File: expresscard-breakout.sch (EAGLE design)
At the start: 3 parts

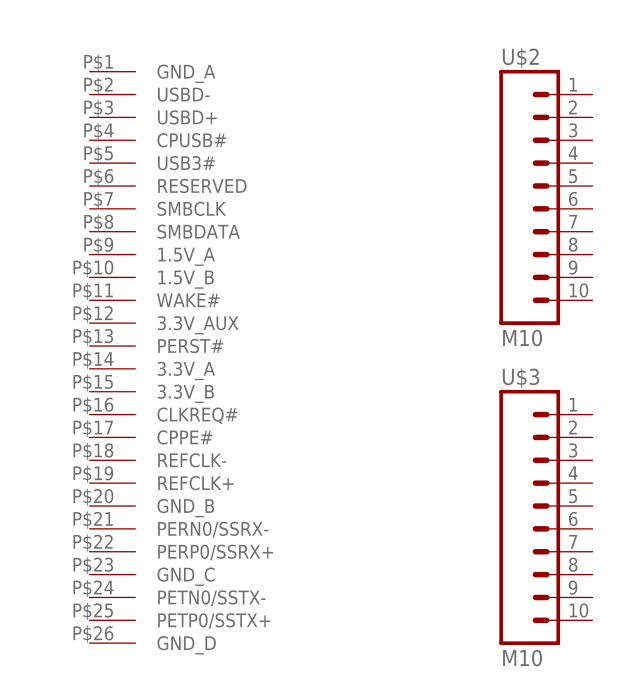
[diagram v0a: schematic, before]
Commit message: I think it is done
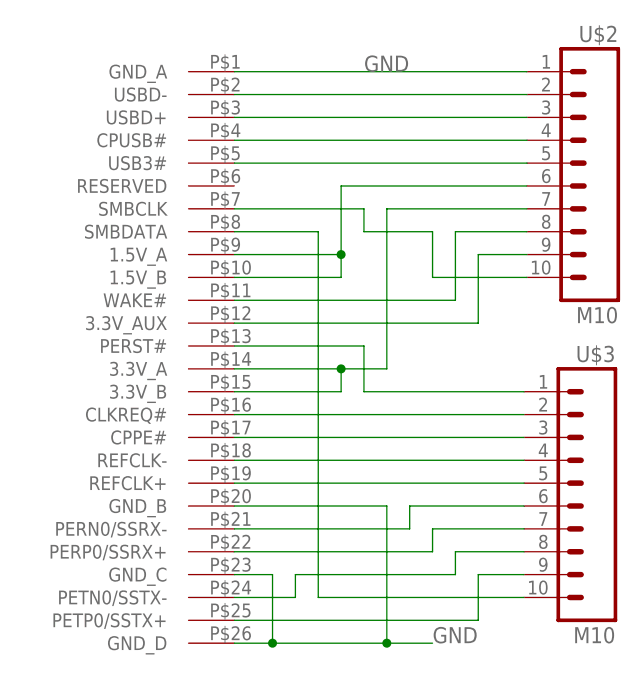
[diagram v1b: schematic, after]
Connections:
- new net GND: U$1.GND_A, U$1.GND_B, U$1.GND_C, U$1.GND_D, U$2.1
- new net N$1: U$1.1.5V_A, U$1.1.5V_B, U$2.6
- new net N$10: U$1.SMBCLK, U$2.10
- new net N$11: U$1.SMBDATA, U$3.10
- new net N$12: U$1.PERST#, U$3.1
- new net N$13: U$1.CLKREQ#, U$3.2
- new net N$14: U$1.CPPE#, U$3.3
- new net N$15: U$1.REFCLK-, U$3.4
- new net N$16: U$1.REFCLK+, U$3.5
- new net N$17: U$1.PERN0/SSRX-, U$3.6
- new net N$18: U$1.PERP0/SSRX+, U$3.7
- new net N$19: U$1.PETN0/SSTX-, U$3.8
- new net N$20: U$1.PETP0/SSTX+, U$3.9
- new net N$3: U$1.USBD-, U$2.2
- new net N$4: U$1.USBD+, U$2.3
- new net N$5: U$1.CPUSB#, U$2.4
- new net N$6: U$1.USB3#, U$2.5
- new net N$7: U$1.3.3V_A, U$1.3.3V_B, U$2.7
- new net N$8: U$1.WAKE#, U$2.8
- new net N$9: U$1.3.3V_AUX, U$2.9
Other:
- moved on the sheet: U$2, U$3
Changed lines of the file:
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@@
 </plain>
 <instances>
-<instance part="U$1" gate="G$1" x="7.62" y="50.8"/>
-<instance part="U$3" gate="G$1" x="58.42" y="30.48"/>
-<instance part="U$2" gate="G$1" x="58.42" y="66.04"/>
+<instance part="U$1" gate="G$1" x="21.1455" y="45.72"/>
+<instance part="U$3" gate="G$1" x="60.96" y="33.02" rot="MR0"/>
+<instance part="U$2" gate="G$1" x="61.2775" y="68.58" rot="MR0"/>
 </instances>
 <busses>
 </busses>
 <nets>
+<net name="GND" class="0">
+<segment>
+<pinref part="U$2" gate="G$1" pin="1"/>
+<wire x1="23.6855" y1="76.2" x2="56.1975" y2="76.2" width="0.1524" layer="91"/>
+<pinref part="U$1" gate="G$1" pin="GND_A"/>
+<label x="38.1" y="76.2" size="1.778" layer="95"/>
+</segment>
+<segment>
+<wire x1="23.6855" y1="27.94" x2="40.64" y2="27.94" width="0.1524" layer="91"/>
+<wire x1="40.64" y1="27.94" x2="40.64" y2="12.7" width="0.1524" layer="91"/>
+<wire x1="23.6855" y1="20.32" x2="27.94" y2="20.32" width="0.1524" layer="91"/>
+<wire x1="27.94" y1="20.32" x2="27.94" y2="12.7" width="0.1524" layer="91"/>
+<wire x1="27.94" y1="12.7" x2="40.64" y2="12.7" width="0.1524" layer="91"/>
+<junction x="40.64" y="12.7"/>
+<junction x="27.94" y="12.7"/>
+<pinref part="U$1" gate="G$1" pin="GND_B"/>
+<pinref part="U$1" gate="G$1" pin="GND_C"/>
+<pinref part="U$1" gate="G$1" pin="GND_D"/>
+<wire x1="23.6855" y1="12.7" x2="27.94" y2="12.7" width="0.1524" layer="91"/>
+<wire x1="40.64" y1="12.7" x2="45.72" y2="12.7" width="0.1524" layer="91"/>
+<label x="45.72" y="12.7" size="1.778" layer="95"/>
+</segment>
+</net>
+<net name="N$3" class="0">
+<segment>
+<wire x1="23.6855" y1="73.66" x2="56.1975" y2="73.66" width="0.1524" layer="91"/>
+<pinref part="U$1" gate="G$1" pin="USBD-"/>
+<pinref part="U$2" gate="G$1" pin="2"/>
+</segment>
+</net>
+<net name="N$4" class="0">
+<segment>
+<wire x1="23.6855" y1="71.12" x2="56.1975" y2="71.12" width="0.1524" layer="91"/>
+<pinref part="U$1" gate="G$1" pin="USBD+"/>
+<pinref part="U$2" gate="G$1" pin="3"/>
+</segment>
+</net>
+<net name="N$5" class="0">
+<segment>
+<pinref part="U$1" gate="G$1" pin="CPUSB#"/>
+<wire x1="23.6855" y1="68.58" x2="56.1975" y2="68.58" width="0.1524" layer="91"/>
+<pinref part="U$2" gate="G$1" pin="4"/>
+</segment>
+</net>
+<net name="N$6" class="0">
+<segment>
+<pinref part="U$1" gate="G$1" pin="USB3#"/>
+<wire x1="23.6855" y1="66.04" x2="56.1975" y2="66.04" width="0.1524" layer="91"/>
+<pinref part="U$2" gate="G$1" pin="5"/>
+</segment>
+</net>
+<net name="N$1" class="0">
+<segment>
+<wire x1="56.1975" y1="63.5" x2="35.56" y2="63.5" width="0.1524" layer="91"/>
+<wire x1="35.56" y1="63.5" x2="35.56" y2="55.88" width="0.1524" layer="91"/>
+<pinref part="U$1" gate="G$1" pin="1.5V_A"/>
+<pinref part="U$2" gate="G$1" pin="6"/>
+<wire x1="35.56" y1="55.88" x2="23.6855" y2="55.88" width="0.1524" layer="91"/>
+<wire x1="23.6855" y1="53.34" x2="35.56" y2="53.34" width="0.1524" layer="91"/>
+<wire x1="35.56" y1="53.34" x2="35.56" y2="55.88" width="0.1524" layer="91"/>
+<junction x="35.56" y="55.88"/>
+<pinref part="U$1" gate="G$1" pin="1.5V_B"/>
+</segment>
+</net>
+<net name="N$7" class="0">
+<segment>
+<wire x1="56.1975" y1="60.96" x2="40.64" y2="60.96" width="0.1524" layer="91"/>
+<wire x1="40.64" y1="60.96" x2="40.64" y2="43.18" width="0.1524" layer="91"/>
+<wire x1="40.64" y1="43.18" x2="35.56" y2="43.18" width="0.1524" layer="91"/>
+<wire x1="35.56" y1="43.18" x2="23.6855" y2="43.18" width="0.1524" layer="91"/>
+<wire x1="23.6855" y1="40.64" x2="35.56" y2="40.64" width="0.1524" layer="91"/>
+<wire x1="35.56" y1="40.64" x2="35.56" y2="43.18" width="0.1524" layer="91"/>
+<junction x="35.56" y="43.18"/>
+<pinref part="U$2" gate="G$1" pin="7"/>
+<pinref part="U$1" gate="G$1" pin="3.3V_A"/>
+<pinref part="U$1" gate="G$1" pin="3.3V_B"/>
+</segment>
+</net>
+<net name="N$8" class="0">
+<segment>
+<wire x1="56.1975" y1="58.42" x2="48.26" y2="58.42" width="0.1524" layer="91"/>
+<wire x1="48.26" y1="58.42" x2="48.26" y2="50.8" width="0.1524" layer="91"/>
+<wire x1="48.26" y1="50.8" x2="23.6855" y2="50.8" width="0.1524" layer="91"/>
+<pinref part="U$2" gate="G$1" pin="8"/>
+<pinref part="U$1" gate="G$1" pin="WAKE#"/>
+</segment>
+</net>
+<net name="N$9" class="0">
+<segment>
+<wire x1="23.6855" y1="48.26" x2="50.8" y2="48.26" width="0.1524" layer="91"/>
+<wire x1="50.8" y1="48.26" x2="50.8" y2="55.88" width="0.1524" layer="91"/>
+<wire x1="50.8" y1="55.88" x2="56.1975" y2="55.88" width="0.1524" layer="91"/>
+<pinref part="U$2" gate="G$1" pin="9"/>
+<pinref part="U$1" gate="G$1" pin="3.3V_AUX"/>
+</segment>
+</net>
+<net name="N$10" class="0">
+<segment>
+<wire x1="23.6855" y1="60.96" x2="38.1" y2="60.96" width="0.1524" layer="91"/>
+<wire x1="38.1" y1="60.96" x2="38.1" y2="58.42" width="0.1524" layer="91"/>
+<wire x1="38.1" y1="58.42" x2="45.72" y2="58.42" width="0.1524" layer="91"/>
+<wire x1="45.72" y1="58.42" x2="45.72" y2="53.34" width="0.1524" layer="91"/>
+<wire x1="45.72" y1="53.34" x2="56.1975" y2="53.34" width="0.1524" layer="91"/>
+<pinref part="U$2" gate="G$1" pin="10"/>
+<pinref part="U$1" gate="G$1" pin="SMBCLK"/>
+</segment>
+</net>
+<net name="N$11" class="0">
+<segment>
+<wire x1="23.6855" y1="58.42" x2="33.02" y2="58.42" width="0.1524" layer="91"/>
+<wire x1="33.02" y1="58.42" x2="33.02" y2="17.78" width="0.1524" layer="91"/>
+<pinref part="U$3" gate="G$1" pin="10"/>
+<wire x1="33.02" y1="17.78" x2="55.88" y2="17.78" width="0.1524" layer="91"/>
+<pinref part="U$1" gate="G$1" pin="SMBDATA"/>
+</segment>
+</net>
+<net name="N$12" class="0">
+<segment>
+<wire x1="23.6855" y1="45.72" x2="38.1" y2="45.72" width="0.1524" layer="91"/>
+<wire x1="38.1" y1="45.72" x2="38.1" y2="40.64" width="0.1524" layer="91"/>
+<pinref part="U$3" gate="G$1" pin="1"/>
+<wire x1="38.1" y1="40.64" x2="55.88" y2="40.64" width="0.1524" layer="91"/>
+<pinref part="U$1" gate="G$1" pin="PERST#"/>
+</segment>
+</net>
+<net name="N$13" class="0">
+<segment>
+<pinref part="U$3" gate="G$1" pin="2"/>
+<pinref part="U$1" gate="G$1" pin="CLKREQ#"/>
+<wire x1="23.6855" y1="38.1" x2="55.88" y2="38.1" width="0.1524" layer="91"/>
+</segment>
+</net>
+<net name="N$14" class="0">
+<segment>
+<pinref part="U$3" gate="G$1" pin="3"/>
+<pinref part="U$1" gate="G$1" pin="CPPE#"/>
+<wire x1="23.6855" y1="35.56" x2="55.88" y2="35.56" width="0.1524" layer="91"/>
+</segment>
+</net>
+<net name="N$15" class="0">
+<segment>
+<pinref part="U$3" gate="G$1" pin="4"/>
+<pinref part="U$1" gate="G$1" pin="REFCLK-"/>
+<wire x1="23.6855" y1="33.02" x2="55.88" y2="33.02" width="0.1524" layer="91"/>
+</segment>
+</net>
+<net name="N$16" class="0">
+<segment>
+<pinref part="U$3" gate="G$1" pin="5"/>
+<pinref part="U$1" gate="G$1" pin="REFCLK+"/>
+<wire x1="23.6855" y1="30.48" x2="55.88" y2="30.48" width="0.1524" layer="91"/>
+</segment>
+</net>
+<net name="N$17" class="0">
+<segment>
+<wire x1="23.6855" y1="25.4" x2="43.18" y2="25.4" width="0.1524" layer="91"/>
+<wire x1="43.18" y1="25.4" x2="43.18" y2="27.94" width="0.1524" layer="91"/>
+<pinref part="U$3" gate="G$1" pin="6"/>
+<wire x1="43.18" y1="27.94" x2="55.88" y2="27.94" width="0.1524" layer="91"/>
+<pinref part="U$1" gate="G$1" pin="PERN0/SSRX-"/>
+</segment>
+</net>
+<net name="N$18" class="0">
+<segment>
+<wire x1="23.6855" y1="22.86" x2="45.72" y2="22.86" width="0.1524" layer="91"/>
+<wire x1="45.72" y1="22.86" x2="45.72" y2="25.4" width="0.1524" layer="91"/>
+<pinref part="U$3" gate="G$1" pin="7"/>
+<wire x1="45.72" y1="25.4" x2="55.88" y2="25.4" width="0.1524" layer="91"/>
+<pinref part="U$1" gate="G$1" pin="PERP0/SSRX+"/>
+</segment>
+</net>
+<net name="N$19" class="0">
+<segment>
+<wire x1="23.6855" y1="17.78" x2="30.48" y2="17.78" width="0.1524" layer="91"/>
+<wire x1="30.48" y1="17.78" x2="30.48" y2="20.32" width="0.1524" layer="91"/>
+<wire x1="30.48" y1="20.32" x2="48.26" y2="20.32" width="0.1524" layer="91"/>
+<wire x1="48.26" y1="20.32" x2="48.26" y2="22.86" width="0.1524" layer="91"/>
+<pinref part="U$3" gate="G$1" pin="8"/>
+<wire x1="48.26" y1="22.86" x2="55.88" y2="22.86" width="0.1524" layer="91"/>
+<pinref part="U$1" gate="G$1" pin="PETN0/SSTX-"/>
+</segment>
+</net>
+<net name="N$20" class="0">
+<segment>
+<wire x1="23.6855" y1="15.24" x2="50.8" y2="15.24" width="0.1524" layer="91"/>
+<wire x1="50.8" y1="15.24" x2="50.8" y2="20.32" width="0.1524" layer="91"/>
+<pinref part="U$3" gate="G$1" pin="9"/>
+<wire x1="50.8" y1="20.32" x2="55.88" y2="20.32" width="0.1524" layer="91"/>
+<pinref part="U$1" gate="G$1" pin="PETP0/SSTX+"/>
+</segment>
+</net>
 </nets>
 </sheet>
